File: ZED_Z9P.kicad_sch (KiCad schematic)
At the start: 42 parts, among them IC2 ZED-F9P-05B, J4 SMA-J-P-X-RA-TH1, Q1 SI1016CX-T1-GE3, Q2 MMBT3904LT1G, Q7 BC849, Q8 BC849, Q9 BC849, U13 LT6000IDCB_TRMPBF, U14 TPS22946YZPR

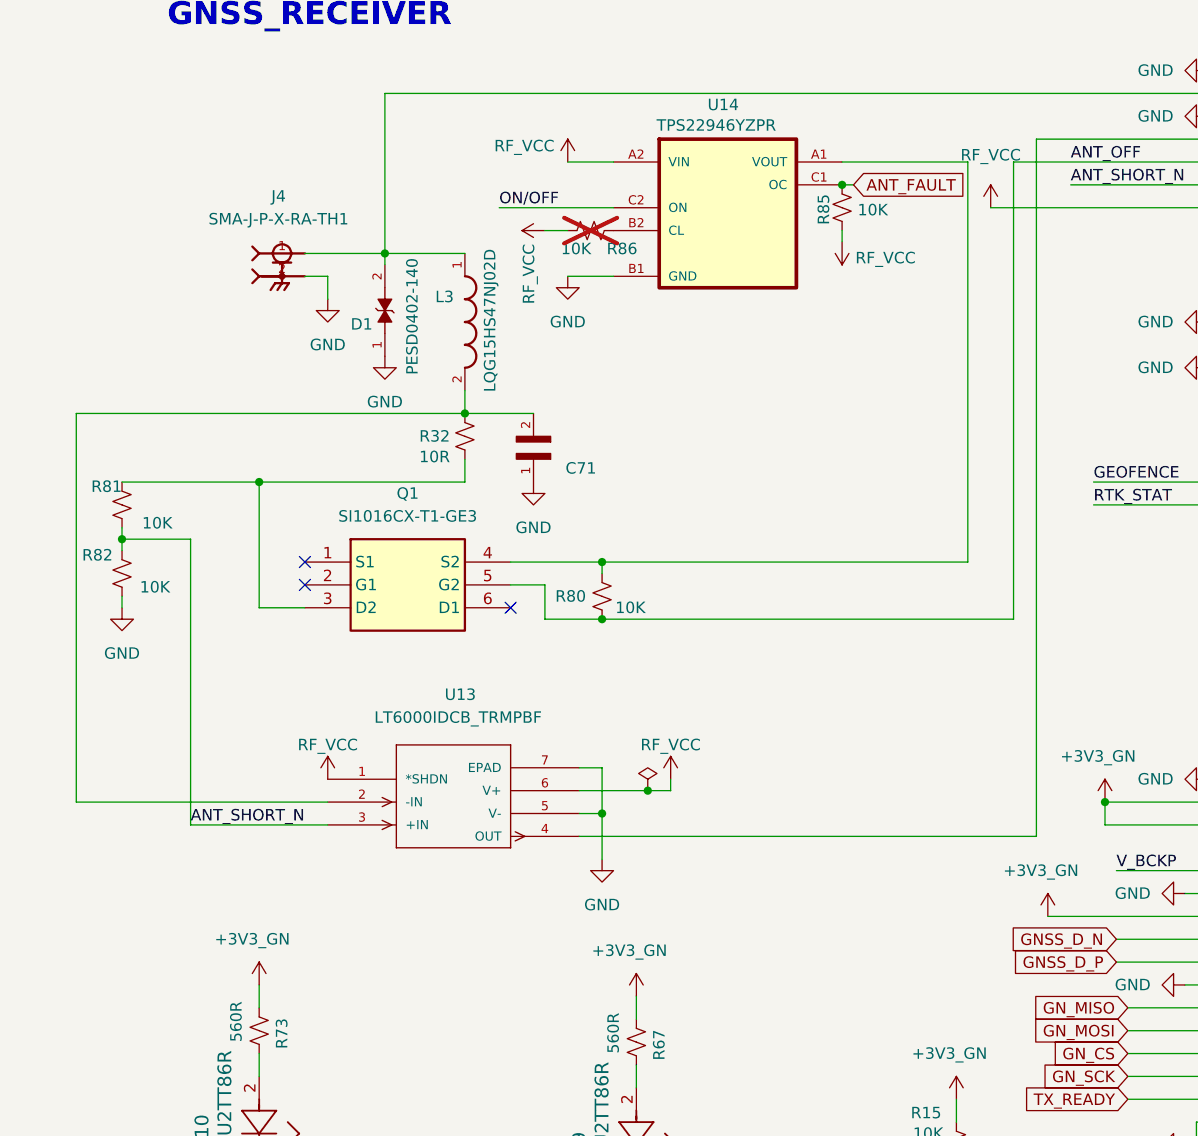
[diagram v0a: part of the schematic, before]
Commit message: new
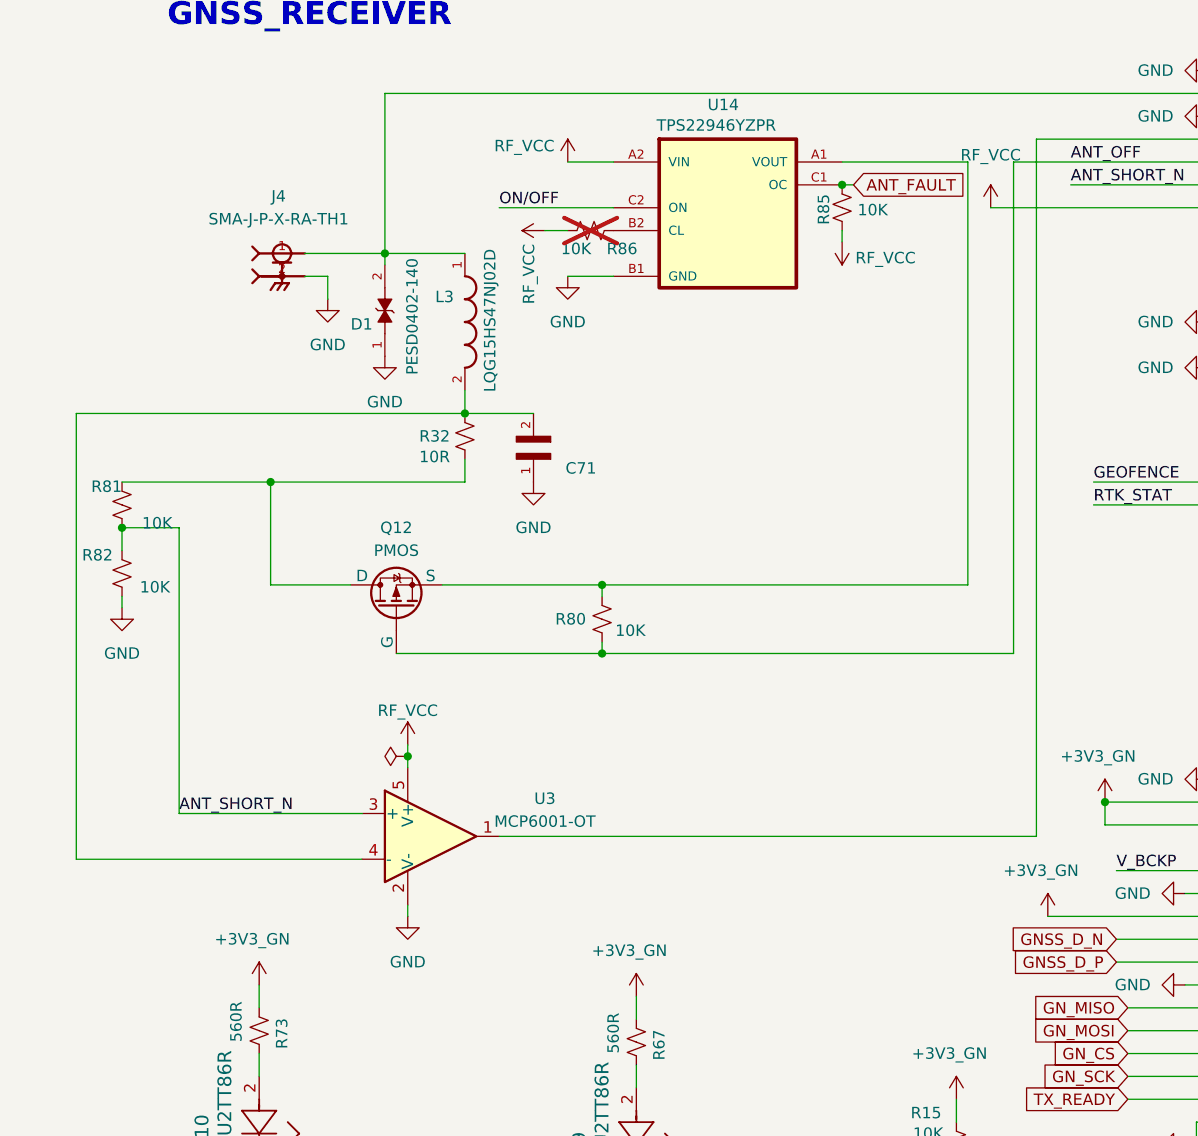
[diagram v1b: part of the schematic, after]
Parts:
- removed Q1: SI1016CX-T1-GE3, GNSS:SOTFL50P160X60-6N, symbol SI1016CX-T1-GE3:SI1016CX-T1-GE3
- removed U13: LT6000IDCB_TRMPBF, GNSS:DFN-6_DCB, symbol LT6000IDCB_TRMPBF:LT6000IDCB_TRMPBF
- added Q12: PMOS, symbol Simulation_SPICE:PMOS
- added U3: MCP6001-OT, Package_TO_SOT_SMD:SOT-23-5, symbol Amplifier_Operational:MCP6001-OT
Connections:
- net ANT_OFF: now also Q12.2 (G)
- net ANT_SHORT_N: now also U3.3 (+)
- net GND: now also U3.2 (V-)
- net RF_VCC: now also U3.5 (V+)
- net at C71.2, L3.2, R32.1: now also U3.4 (-)
- net at IC2.4 (ANT_DETECT): now also U3.1
- net at R32.2, R81.2: now also Q12.1 (D)
- net at R80.2, U14.A1 (VOUT): now also Q12.3 (S)
- no-connect marks 26 -> 23
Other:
- moved on the sheet: R80
